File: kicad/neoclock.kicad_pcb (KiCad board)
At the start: 2 copper layers, 58.2 x 41.9 mm, 26 parts, among them CON1 2.1mm 5V, IC1 ATMEGA328P-A, K1 NEOPIXEL, P1 ICSP, P2 FTDI, SW1 HOUR, SW2 MINUTE, U1 DS1307, X1 16Mhz, X2 32.768kHz

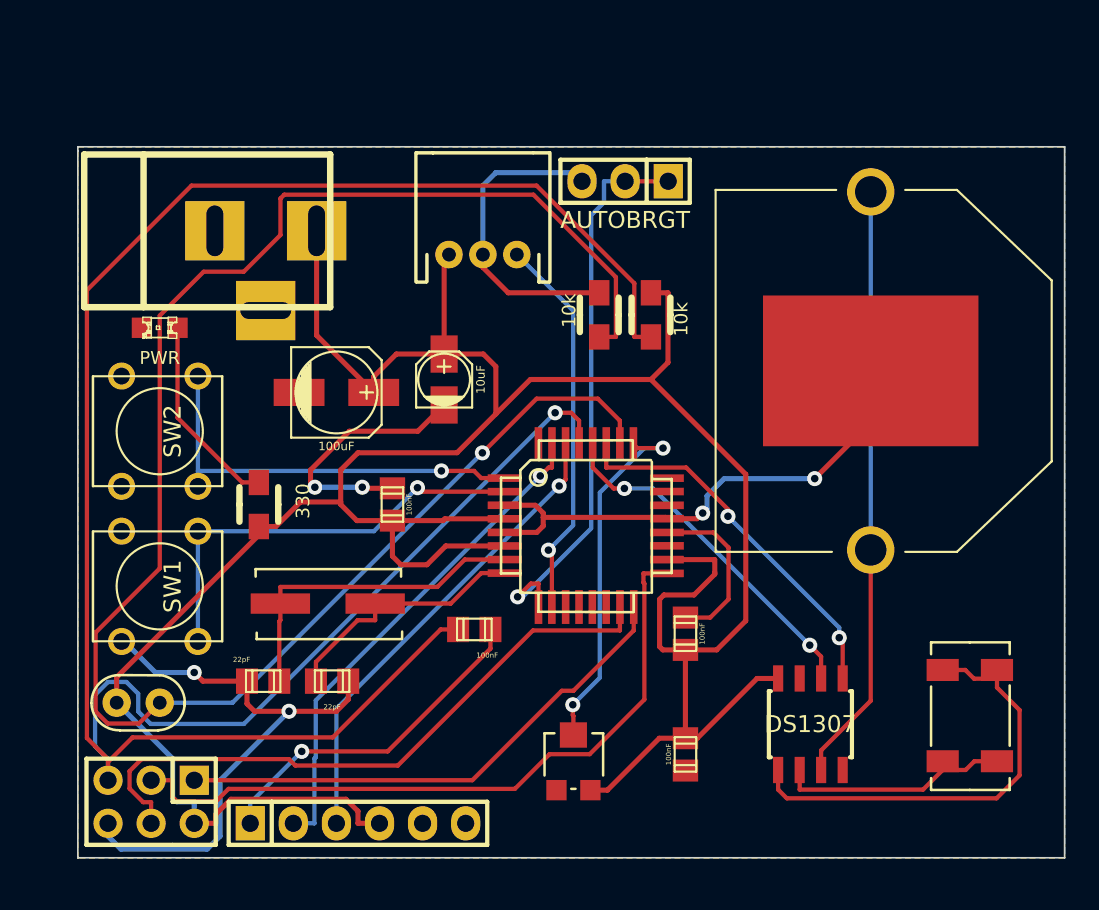
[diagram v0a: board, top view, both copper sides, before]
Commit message: updating pcb finally
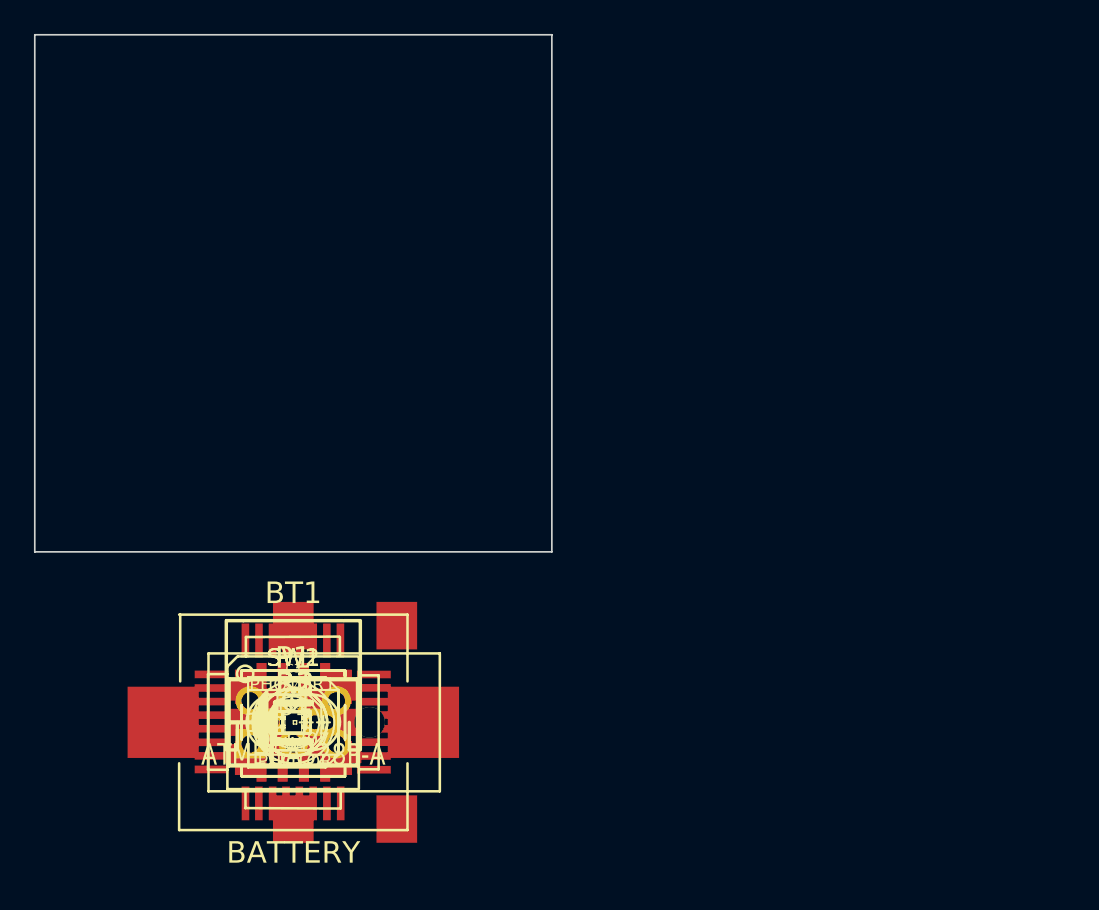
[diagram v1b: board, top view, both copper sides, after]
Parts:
- removed C8: 100nF, Capacitors_SMD:c_0805
- removed JP1: AUTOBRGT, Pin_Headers:Pin_Header_Straight_1x03
- removed P2: FTDI, Pin_Headers:Pin_Header_Straight_1x06
- removed RV1: POT, synic:Timmer_Pot_ST32ETA103
- BT1: footprint synic:WNL_CR2302_TH_KEYSTONE_3003 -> synic:BK-755_12mm_coincell
- CON1: footprint Connect:BARREL_JACK -> synic:BARREL_JACK_SMD
- K1: footprint jst-3-pth-ra -> synic:jst-3-pth-ra
- PHOTOR1: footprint PHOTORESISTOR -> synic:PHOTORESISTOR
- SW1, SW2: footprint synic:SW_PUSH_SMALL -> synic:SMD_PUSHBUTTON_MINI
- U1: footprint SOIC8:Test -> SOIC_Packages:SOIC-8_N
- X1: footprint synic:Crystal_HC49-SMALL_SMD -> synic:4padCrystalSMD_7.0x5.0mm
- X2: footprint Crystal-4pad -> synic:4padCrystalSMD_7.0x5.0mm
- moved X2 39.9 mm to (34.3, 57.0), turned to 0 degrees
- moved BT1 39.8 mm to (34.3, 57.0), turned to 0 degrees
- moved R2 32.0 mm to (34.3, 57.0), turned to 0 degrees
- moved U1 30.5 mm to (34.3, 57.0)
- moved R3 30.0 mm to (34.3, 57.0), turned to 0 degrees
- moved K1 29.8 mm to (34.3, 57.0)
- moved CON1 29.4 mm to (34.3, 57.0)
- moved D1 24.6 mm to (34.3, 57.0), turned to 0 degrees
- moved C2 23.7 mm to (34.3, 57.0), turned to 0 degrees
- moved C1 23.2 mm to (34.3, 57.0), turned to 0 degrees
- moved C4 22.1 mm to (34.3, 57.0), turned to 0 degrees
- moved IC1 20.8 mm to (34.3, 57.0)
- moved C3 19.6 mm to (34.3, 57.0)
- moved SW2 18.9 mm to (34.3, 57.0), turned to 0 degrees
- moved C7 14.1 mm to (34.3, 57.0), turned to 0 degrees
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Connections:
- IC1 pad 25: BRIGHTNESS -> Net-(IC1-Pad25)
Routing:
- net VCC: track 170.9 -> 0.00 mm
- net Net-(IC1-Pad29): track 139.6 -> 0.00 mm, vias 1 -> 0
- net Net-(IC1-Pad26): track 103.6 -> 0.00 mm, vias 1 -> 0
- net GND: track 99.0 -> 0.00 mm, vias 6 -> 0
- net Net-(IC1-Pad17): track 41.5 -> 0.00 mm
- net Net-(IC1-Pad15): track 37.9 -> 0.00 mm
- net Net-(BT1-Pad1): track 35.3 -> 0.00 mm
- net Net-(IC1-Pad9): track 33.5 -> 0.00 mm, vias 1 -> 0
- net Net-(IC1-Pad16): track 30.9 -> 0.00 mm
- net FTDI2: track 29.5 -> 0.00 mm, vias 1 -> 0
- net FTDI3: track 27.9 -> 0.00 mm, vias 1 -> 0
- net Net-(U1-Pad1): track 26.3 -> 0.00 mm
- net Net-(IC1-Pad2): track 25.7 -> 0.00 mm, vias 1 -> 0
- net Net-(IC1-Pad1): track 24.8 -> 0.00 mm, vias 1 -> 0
- net Net-(IC1-Pad10): track 22.8 -> 0.00 mm, vias 1 -> 0
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- removed copper zone on B.Cu, net GND
- removed copper zone on F.Cu, net GND
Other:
- board size 58.2 x 41.9 mm -> 30.5 x 30.5 mm
- net class VCC removed
- rule trace_min: 0.2 -> 0.254
- board text removed: "NeoClock v0 by Adam Olsen arolsen@gmail.com"

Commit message: woot
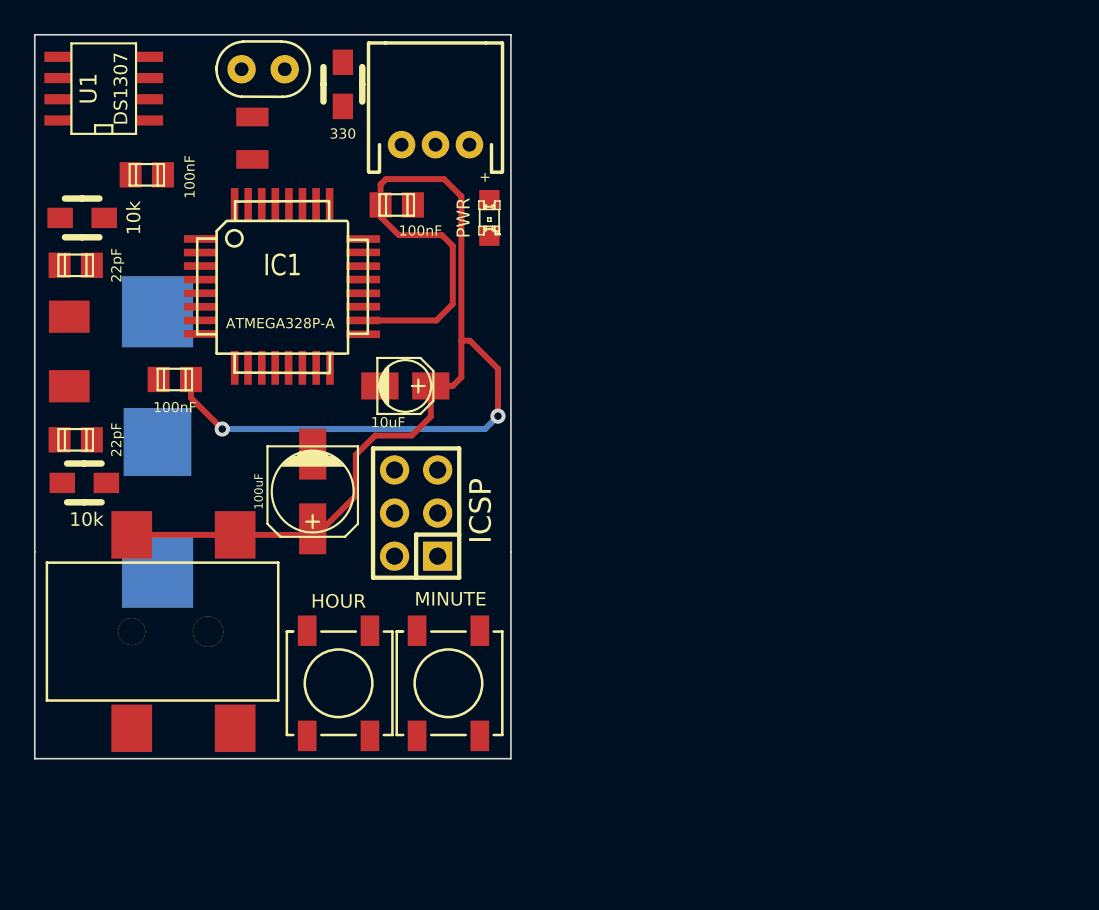
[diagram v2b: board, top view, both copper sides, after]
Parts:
- BT1: moved to B.Cu
- X1: footprint synic:4padCrystalSMD_7.0x5.0mm -> synic:2_SMD_CRYSTAL_5.0x3.20
- X2: footprint synic:4padCrystalSMD_7.0x5.0mm -> synic:2_SMD_CRYSTAL_3.2x1.5
- moved U1 39.0 mm to (23.1, 19.7), turned to 90 degrees
- moved PHOTOR1 38.5 mm to (32.5, 18.5), turned to 180 degrees
- moved R1 37.7 mm to (37.2, 19.4), turned to 270 degrees
- moved K1 35.1 mm to (42.7, 23.0)
- moved X2 34.5 mm to (31.9, 22.6), turned to 270 degrees
- moved C7 33.4 mm to (25.7, 24.8)
- moved R2 32.2 mm to (21.8, 27.3)
- moved D1 31.9 mm to (45.8, 27.3), turned to 270 degrees
- moved C2 31.1 mm to (40.4, 26.5)
- moved C5 29.8 mm to (21.5, 30.1)
- moved IC1 25.7 mm to (33.7, 31.4)
- moved X1 25.5 mm to (21.1, 35.2), turned to 270 degrees
- moved C1 21.4 mm to (27.3, 36.8), turned to 180 degrees
- moved C6 21.0 mm to (21.5, 40.4)
- moved C4 20.9 mm to (40.9, 37.2)
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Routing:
- net VCC: track 0.00 -> 83.6 mm, vias 0 -> 2
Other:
- board size 30.5 x 30.5 mm -> 28.1 x 42.7 mm
- net class POWER added: clearance 0.254, trace_width 0.35, via_dia 0.889, via_drill 0.635
- board text added: "+"
